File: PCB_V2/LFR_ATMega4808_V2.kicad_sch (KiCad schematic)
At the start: 72 parts, among them J1 Conn_02x02_Odd_Even, J2 Conn_02x05_Odd_Even, J3 Conn_02x02_Counter_Clockwise, J4 Conn_02x02_Counter_Clockwise, J5 Conn_02x02_Counter_Clockwise, J6 Conn_02x03_Odd_Even, J7 Conn_02x02_Odd_Even, Q1 PMOS, Q2 NMOS, Q3 NMOS, Q4 NMOS, Q5 NMOS, Q6 PMOS, Q7 NMOS, Q8 NMOS, U1 ATmega4808-A, U5 MCP1700x-330xxTO

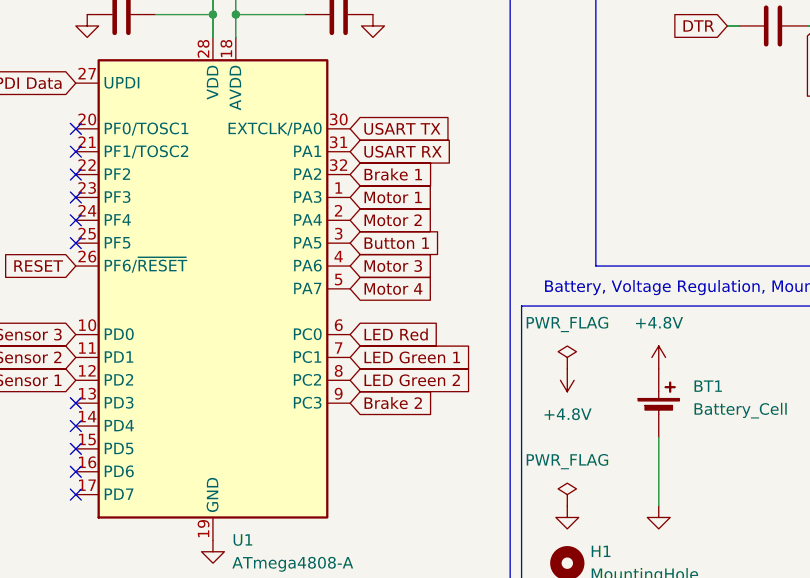
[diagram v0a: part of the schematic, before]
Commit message: Everything except for buttons is done
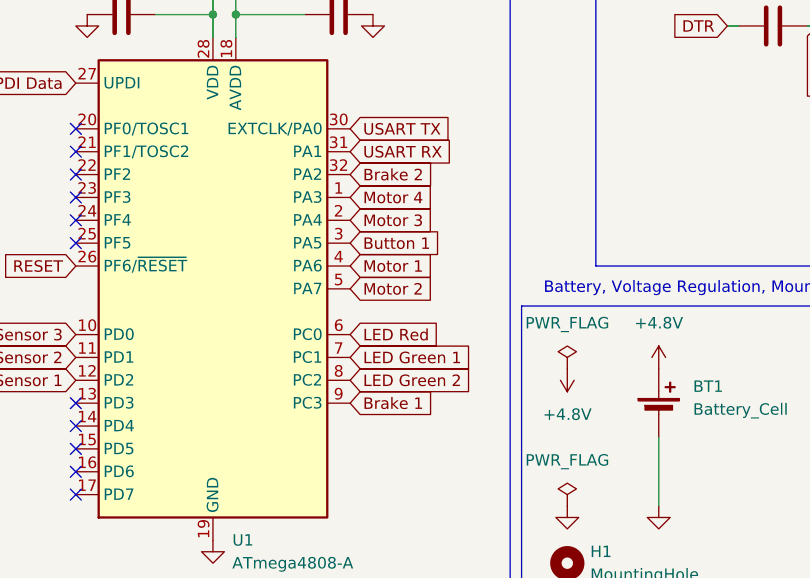
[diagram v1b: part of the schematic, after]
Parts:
- S2, S4: footprint MJTP1230:SW_MJTP1230 -> MJTP1230_:Switch_Tactile_THT_6x6mm_MJTP1230
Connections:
- net Brake 1: now also U1.9 (PC3); no longer U1.32 (PA2)
- net Brake 2: now also U1.32 (PA2); no longer U1.9 (PC3)
- net Motor 1: now also U1.4 (PA6); no longer U1.1 (PA3)
- net Motor 2: now also U1.5 (PA7); no longer U1.2 (PA4)
- net Motor 3: now also U1.2 (PA4); no longer U1.4 (PA6)
- net Motor 4: now also U1.1 (PA3); no longer U1.5 (PA7)
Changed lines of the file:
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@@
 	(global_label "Motor 3"
 		(shape input)
-		(at 64.77 53.34 0)
+		(at 64.77 48.26 0)
 		(fields_autoplaced yes)
 		(effects
@@
 		)
 		(property "Intersheetrefs" "${INTERSHEET_REFS}"
-			(at 75.1936 53.34 0)
+			(at 75.1936 48.26 0)
 			(hide yes)
 			(show_name no)
@@
 	(global_label "Motor 4"
 		(shape input)
-		(at 64.77 55.88 0)
+		(at 64.77 45.72 0)
 		(fields_autoplaced yes)
 		(effects
@@
 		)
 		(property "Intersheetrefs" "${INTERSHEET_REFS}"
-			(at 75.1936 55.88 0)
+			(at 75.1936 45.72 0)
 			(hide yes)
 			(show_name no)
@@
 	(global_label "Motor 1"
 		(shape input)
-		(at 64.77 45.72 0)
+		(at 64.77 53.34 0)
 		(fields_autoplaced yes)
 		(effects
@@
 		)
 		(property "Intersheetrefs" "${INTERSHEET_REFS}"
-			(at 75.1936 45.72 0)
+			(at 75.1936 53.34 0)
 			(hide yes)
 			(show_name no)
@@
 	(global_label "Brake 1"
 		(shape input)
-		(at 64.77 43.18 0)
+		(at 64.77 68.58 0)
 		(fields_autoplaced yes)
 		(effects
@@
 		)
 		(property "Intersheetrefs" "${INTERSHEET_REFS}"
-			(at 75.2542 43.18 0)
+			(at 75.2542 68.58 0)
 			(hide yes)
 			(show_name no)
@@
 	(global_label "Motor 2"
 		(shape input)
-		(at 64.77 48.26 0)
+		(at 64.77 55.88 0)
 		(fields_autoplaced yes)
 		(effects
@@
 		)
 		(property "Intersheetrefs" "${INTERSHEET_REFS}"
-			(at 75.1936 48.26 0)
+			(at 75.1936 55.88 0)
 			(hide yes)
 			(show_name no)
@@
 	(global_label "Brake 2"
 		(shape input)
-		(at 64.77 68.58 0)
+		(at 64.77 43.18 0)
 		(fields_autoplaced yes)
 		(effects
@@
 		)
 		(property "Intersheetrefs" "${INTERSHEET_REFS}"
-			(at 75.2542 68.58 0)
+			(at 75.2542 43.18 0)
 			(hide yes)
 			(show_name no)
@@
 			)
 		)
-		(property "Footprint" "MJTP1230:SW_MJTP1230"
+		(property "Footprint" "MJTP1230_:Switch_Tactile_THT_6x6mm_MJTP1230"
 			(at 39.37 167.64 0)
 			(hide yes)
@@
 			)
 		)
-		(property "Footprint" "MJTP1230:SW_MJTP1230"
+		(property "Footprint" "MJTP1230_:Switch_Tactile_THT_6x6mm_MJTP1230"
 			(at 133.35 38.1 0)
 			(hide yes)

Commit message: Finished the wiring, now on to the silkscreen
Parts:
- H1, H2, H3, H4: footprint MountingHole:MountingHole_2.2mm_M2 -> MountingHole:MountingHole_2.2mm_M2_Pad
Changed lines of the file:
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@@
 			)
 		)
-		(property "Footprint" "MountingHole:MountingHole_2.2mm_M2"
+		(property "Footprint" "MountingHole:MountingHole_2.2mm_M2_Pad"
 			(at 88.9 101.6 0)
 			(hide yes)
@@
 			)
 		)
-		(property "Footprint" "MountingHole:MountingHole_2.2mm_M2"
+		(property "Footprint" "MountingHole:MountingHole_2.2mm_M2_Pad"
 			(at 88.9 86.36 0)
 			(hide yes)
@@
 			)
 		)
-		(property "Footprint" "MountingHole:MountingHole_2.2mm_M2"
+		(property "Footprint" "MountingHole:MountingHole_2.2mm_M2_Pad"
 			(at 88.9 96.52 0)
 			(hide yes)
@@
 			)
 		)
-		(property "Footprint" "MountingHole:MountingHole_2.2mm_M2"
+		(property "Footprint" "MountingHole:MountingHole_2.2mm_M2_Pad"
 			(at 88.9 91.44 0)
 			(hide yes)
